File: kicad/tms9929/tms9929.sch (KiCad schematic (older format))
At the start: 47 parts, among them U1 TMS9929A, U2 4164, U3 4164

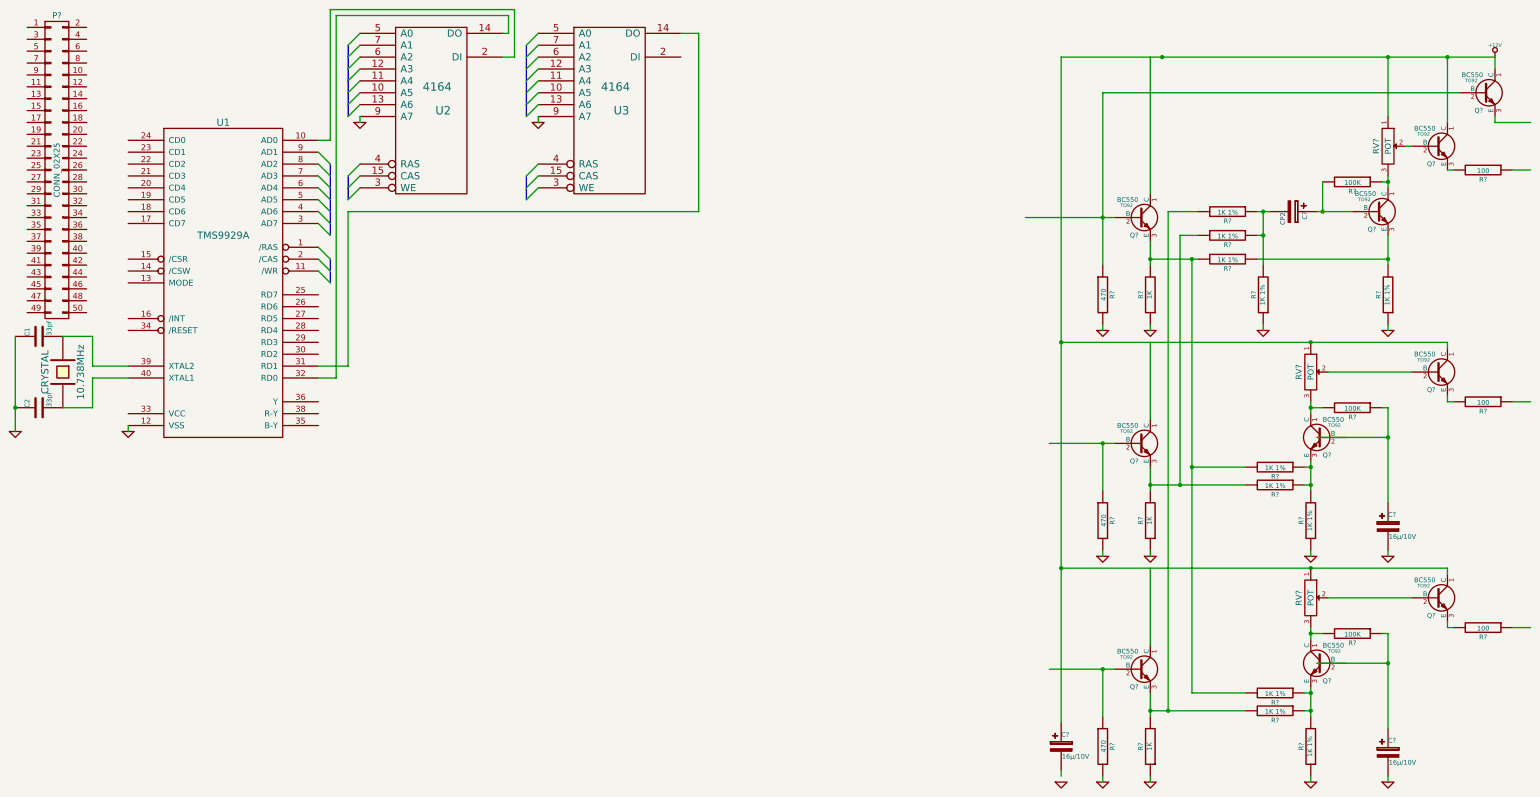
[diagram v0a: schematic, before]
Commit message: A1 an DI
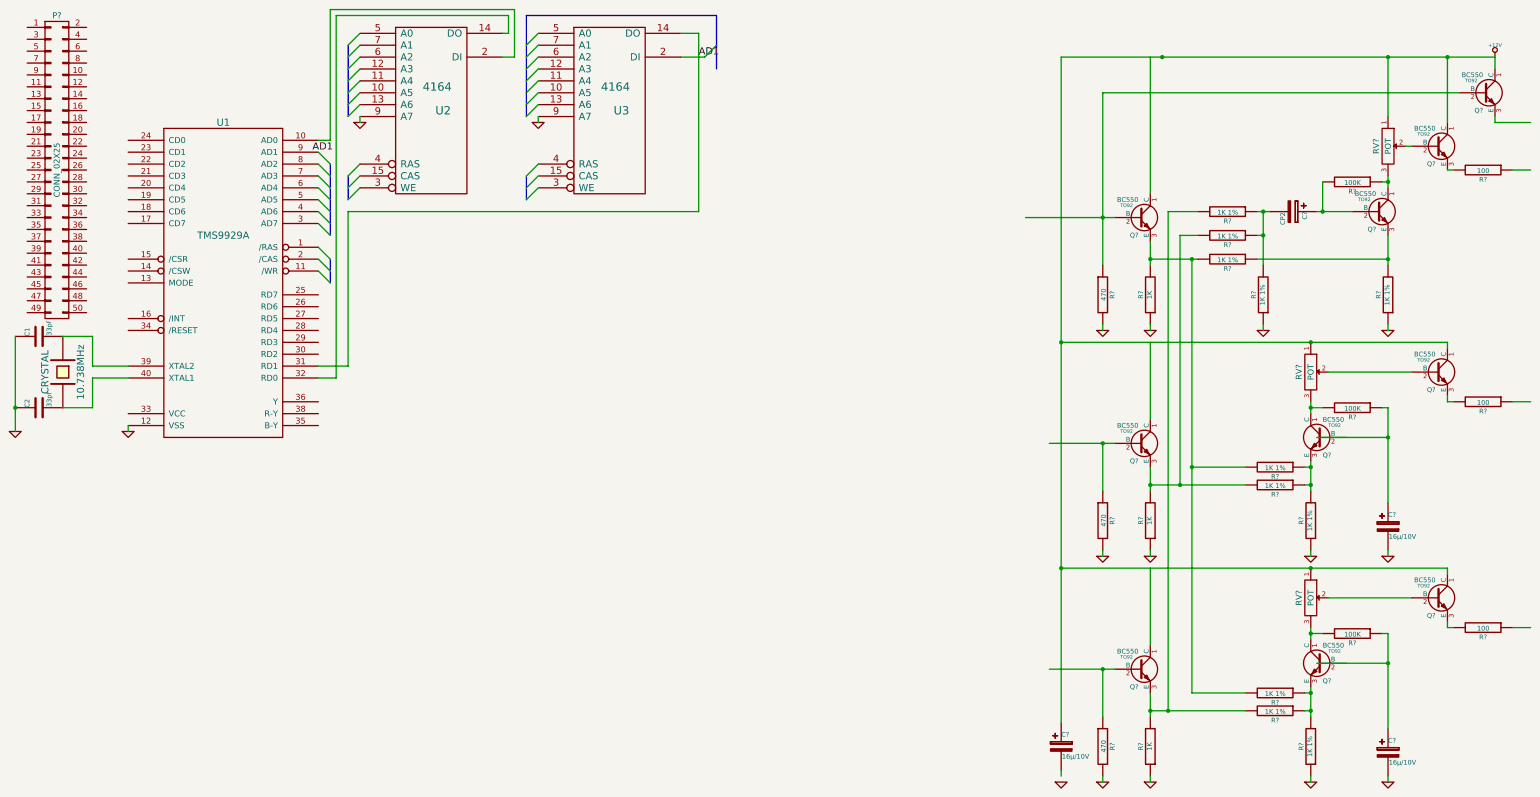
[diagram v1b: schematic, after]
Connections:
- net labels added: AD1
- wire segments 140 -> 109
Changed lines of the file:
@@
 	5100 2150 5200 2050
 Wire Bus Line
-	3450 1850 3450 1950
-Wire Bus Line
-	3450 1950 3450 2050
-Wire Bus Line
-	3450 2050 3450 2150
-Wire Bus Line
-	3450 2150 3450 2250
-Wire Bus Line
-	3450 2250 3450 2350
-Wire Bus Line
-	3450 2350 3450 2450
-Wire Bus Line
-	3600 850  3600 950
-Wire Bus Line
-	3600 950  3600 1050
-Wire Bus Line
-	3600 1050 3600 1150
-Wire Bus Line
-	3600 1150 3600 1250
-Wire Bus Line
-	3600 1250 3600 1350
-Wire Bus Line
-	3600 1350 3600 1450
+	3450 1850 3450 2450
+Wire Bus Line
+	3600 850  3600 1450
 Wire Wire Line
 	3700 1450 3700 1500
 Wire Bus Line
-	3450 2650 3450 2750
-Wire Bus Line
-	3450 2750 3450 2850
-Wire Bus Line
-	3600 1950 3600 2050
-Wire Bus Line
-	3600 2050 3600 2150
+	3450 2650 3450 2850
+Wire Bus Line
+	3600 1950 3600 2150
 Wire Wire Line
 	1750 3650 1450 3650
@@
 	1750 4050 1750 4100
 Wire Wire Line
-	800  3300 800  3900
-Wire Wire Line
-	800  3900 800  4100
+	800  3300 800  4100
 Connection ~ 800  3900
 Wire Wire Line
 	12550 1700 12500 1700
 Wire Wire Line
-	12350 1950 12350 2000
-Wire Wire Line
-	12350 2000 12350 2050
+	12350 1950 12350 2050
 Connection ~ 12350 2000
 Wire Wire Line
-	11750 2250 11800 2250
-Wire Wire Line
-	11800 2250 12050 2250
+	11750 2250 12050 2250
 Wire Wire Line
 	12300 2000 12350 2000
@@
 Connection ~ 11800 2250
 Wire Wire Line
-	11250 2250 11300 2250
-Wire Wire Line
-	11300 2250 11350 2250
-Wire Wire Line
-	11300 2250 11300 2450
-Wire Wire Line
-	11300 2450 11300 2700
+	11250 2250 11350 2250
+Wire Wire Line
+	11300 2250 11300 2700
 Connection ~ 11300 2250
 Wire Wire Line
@@
 	11250 2650 12350 2650
 Wire Wire Line
-	12350 2450 12350 2650
-Wire Wire Line
-	12350 2650 12350 2700
+	12350 2450 12350 2700
 Connection ~ 12350 2650
 Wire Wire Line
@@
 	12850 950  12850 1500
 Wire Wire Line
-	9600 950  10450 950
-Wire Wire Line
-	10450 950  12350 950
-Wire Wire Line
-	12350 950  12850 950
-Wire Wire Line
-	12850 950  13250 950
+	9600 950  13250 950
 Wire Wire Line
 	12850 1900 12900 1900
@@
 	11800 3900 11700 3900
 Wire Wire Line
-	11700 3850 11700 3900
-Wire Wire Line
-	11700 3900 11700 3950
+	11700 3850 11700 3950
 Wire Wire Line
 	12850 3350 12850 3400
@@
 	11850 3600 12550 3600
 Wire Wire Line
-	12350 3900 12350 4150
-Wire Wire Line
-	12350 4150 12350 4700
+	12350 3900 12350 4700
 Wire Wire Line
 	11750 4150 12350 4150
 Wire Wire Line
-	11700 4350 11700 4400
-Wire Wire Line
-	11700 4400 11700 4550
-Wire Wire Line
-	11700 4550 11700 4600
+	11700 4350 11700 4600
 Wire Wire Line
 	11650 4550 11700 4550
@@
 Connection ~ 11700 3350
 Wire Wire Line
-	10350 4550 10600 4550
-Wire Wire Line
-	10600 4550 11150 4550
-Wire Wire Line
-	10350 4400 10350 4550
-Wire Wire Line
-	10350 4550 10350 4600
+	10350 4550 11150 4550
+Wire Wire Line
+	10350 4400 10350 4600
 Connection ~ 10350 4550
 Wire Wire Line
 	9950 4600 9950 4200
 Wire Wire Line
-	9500 4200 9950 4200
-Wire Wire Line
-	9950 4200 10050 4200
+	9500 4200 10050 4200
 Wire Wire Line
 	12350 5100 12350 5150
@@
 	11800 5800 11700 5800
 Wire Wire Line
-	11700 5750 11700 5800
-Wire Wire Line
-	11700 5800 11700 5850
+	11700 5750 11700 5850
 Wire Wire Line
 	12850 5250 12850 5300
@@
 	11850 5500 12550 5500
 Wire Wire Line
-	12350 5800 12350 6050
-Wire Wire Line
-	12350 6050 12350 6600
+	12350 5800 12350 6600
 Wire Wire Line
 	11750 6050 12350 6050
 Wire Wire Line
-	11700 6250 11700 6300
-Wire Wire Line
-	11700 6300 11700 6450
-Wire Wire Line
-	11700 6450 11700 6500
+	11700 6250 11700 6500
 Wire Wire Line
 	11650 6450 11700 6450
@@
 Connection ~ 11700 5250
 Wire Wire Line
-	10350 6450 10500 6450
-Wire Wire Line
-	10500 6450 11150 6450
-Wire Wire Line
-	10350 6300 10350 6450
-Wire Wire Line
-	10350 6450 10350 6500
+	10350 6450 11150 6450
+Wire Wire Line
+	10350 6300 10350 6500
 Connection ~ 10350 6450
 Wire Wire Line
 	9950 6500 9950 6100
 Wire Wire Line
-	9500 6100 9950 6100
-Wire Wire Line
-	9950 6100 10050 6100
+	9500 6100 10050 6100
 Wire Wire Line
 	12350 7000 12350 7050
@@
 	12850 5700 12850 5750
 Wire Wire Line
-	9600 5250 11700 5250
-Wire Wire Line
-	11700 5250 12850 5250
-Wire Wire Line
-	9600 950  9600 3350
-Wire Wire Line
-	9600 3350 9600 5250
-Wire Wire Line
-	9600 5250 9600 6550
+	9600 5250 12850 5250
+Wire Wire Line
+	9600 950  9600 6550
 Connection ~ 9600 3350
 Connection ~ 9600 5250
@@
 	10350 950  10350 2100
 Wire Wire Line
-	10350 2500 10350 2650
-Wire Wire Line
-	10350 2650 10350 2700
-Wire Wire Line
-	9950 1250 9950 2300
-Wire Wire Line
-	9950 2300 9950 2700
-Wire Wire Line
-	9300 2300 9950 2300
-Wire Wire Line
-	9950 2300 10050 2300
+	10350 2500 10350 2700
+Wire Wire Line
+	9950 1250 9950 2700
+Wire Wire Line
+	9300 2300 10050 2300
 Wire Wire Line
 	10350 3200 10350 3250
@@
 	12350 3200 12350 3250
 Wire Wire Line
-	10350 2650 10700 2650
-Wire Wire Line
-	10700 2650 10750 2650
+	10350 2650 10750 2650
 Connection ~ 10350 2650
 Connection ~ 10450 950
@@
 	11150 4400 10700 4400
 Wire Wire Line
-	10700 2650 10700 4400
-Wire Wire Line
-	10700 4400 10700 6300
+	10700 2650 10700 6300
 Connection ~ 10700 2650
 Wire Wire Line
@@
 	10350 5900 10350 5250
 Wire Wire Line
-	9600 3350 11700 3350
-Wire Wire Line
-	11700 3350 12850 3350
+	9600 3350 12850 3350
 Wire Wire Line
 	10750 2250 10500 2250
@@
 Connection ~ 9950 6100
 Wire Bus Line
-	5100 850  5100 950
-Wire Bus Line
-	5100 950  5100 1050
-Wire Bus Line
-	5100 1050 5100 1150
-Wire Bus Line
-	5100 1150 5100 1250
-Wire Bus Line
-	5100 1250 5100 1350
-Wire Bus Line
-	5100 1350 5100 1450
+	5100 600  5100 1450
 Wire Wire Line
 	5200 1450 5200 1500
 Wire Bus Line
-	5100 1950 5100 2050
-Wire Bus Line
-	5100 2050 5100 2150
+	5100 1950 5100 2150
 Wire Wire Line
 	3350 3650 3500 3650
@@
 	3600 3550 3600 2250
 Wire Wire Line
-	6550 2250 3600 2250
-Wire Wire Line
-	6550 750  6550 2250
+	3600 2250 6550 2250
+Wire Wire Line
+	6550 2250 6550 750
 Wire Wire Line
 	6550 750  6400 750
@@
 	1    0    0    -1
 $EndComp
+Wire Bus Line
+	5100 600  6700 600
+Wire Bus Line
+	6700 600  6700 1050
+Entry Wire Line
+	6600 950  6700 850
+Wire Wire Line
+	6400 950  6600 950
+Text Label 6550 950  0    60   ~ 0
+AD1
+Text Label 3300 1750 0    60   ~ 0
+AD1
 $EndSCHEMATC
